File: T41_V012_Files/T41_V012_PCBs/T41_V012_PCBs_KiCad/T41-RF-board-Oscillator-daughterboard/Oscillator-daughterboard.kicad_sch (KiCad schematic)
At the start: 26 parts, among them J2 pin header, J3 pin header, J4 pin header, J5 OEBSSEN, U1 Si5351A-B-GM, U2 SY10EP51VKG, U3 SY10EP51VKG, U4 SY10EP51VKG, U5 SY10EP51VKG, U6 SY10EP51VKG, Y1 ECS-TX053-S3

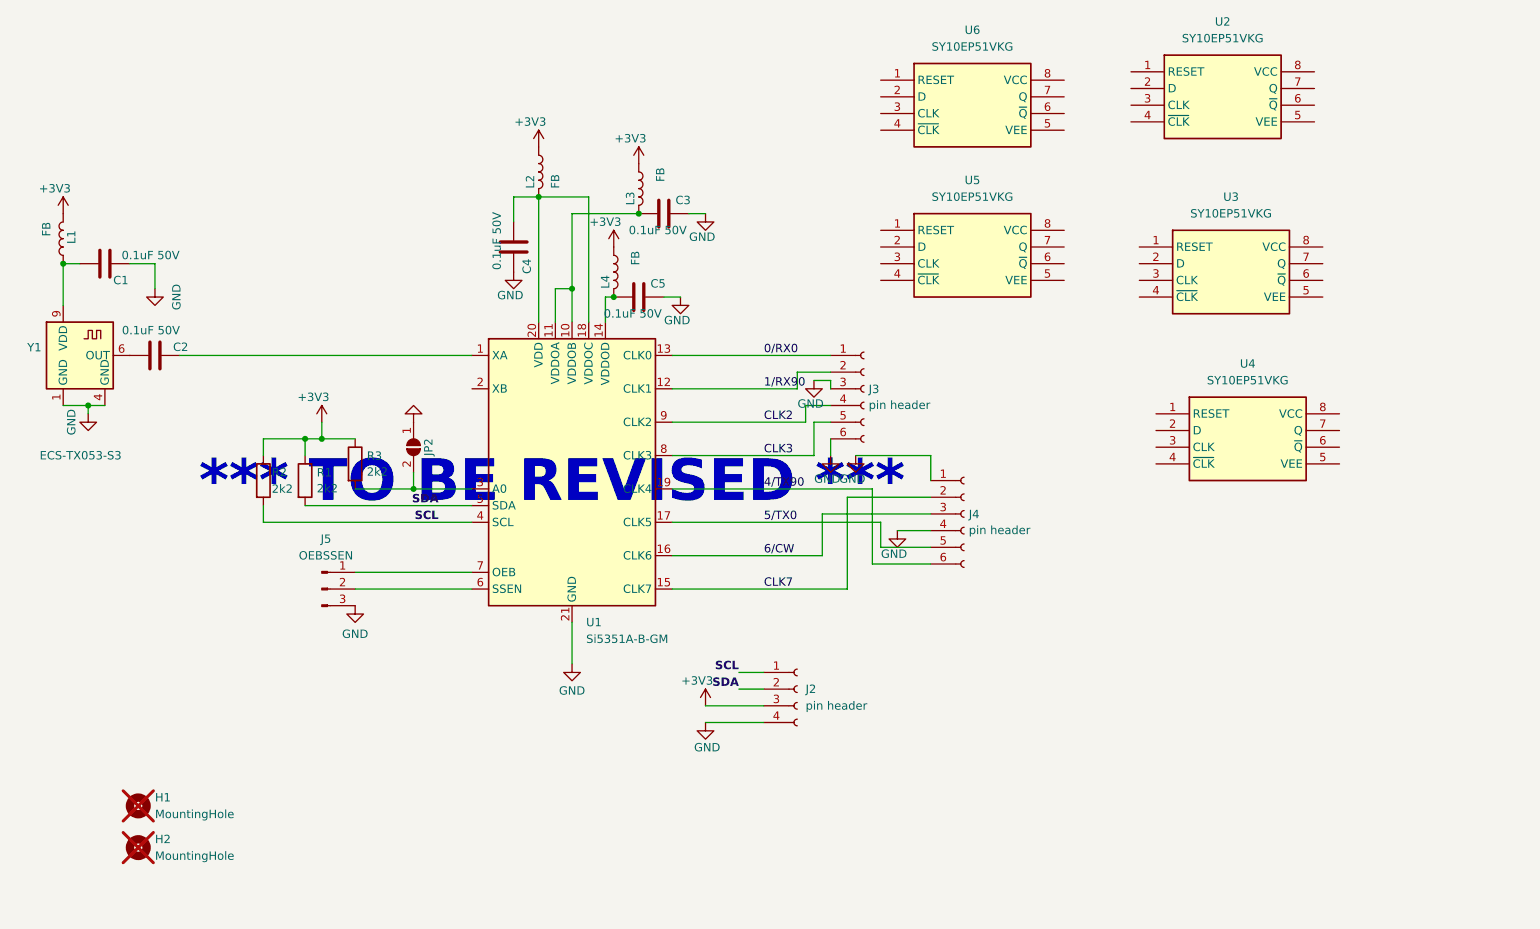
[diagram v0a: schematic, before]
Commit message: File updates
file updates
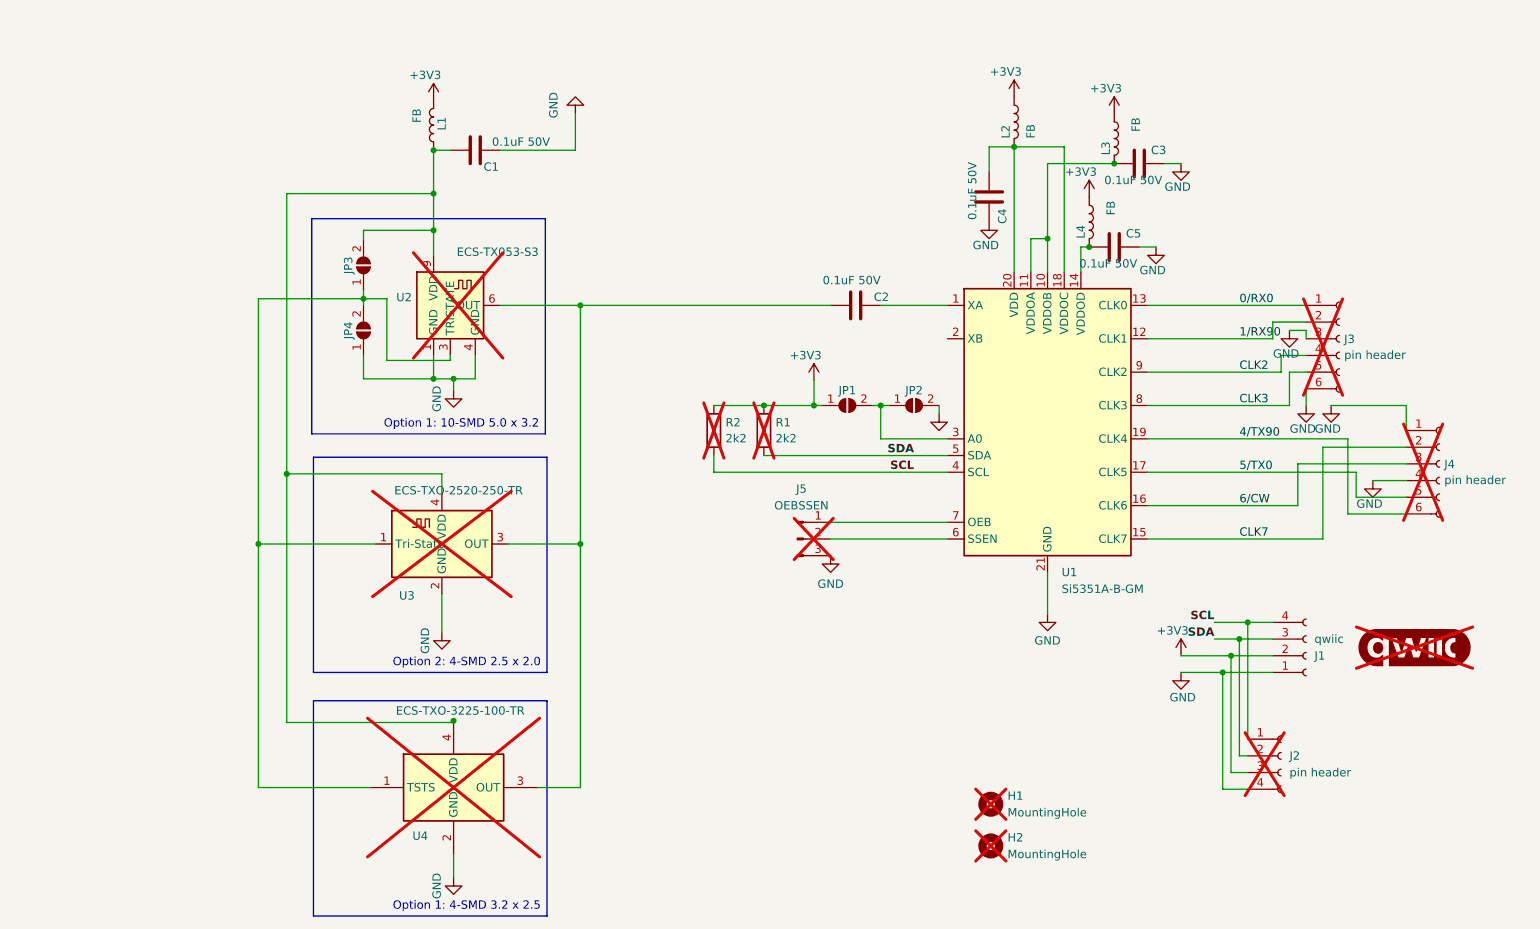
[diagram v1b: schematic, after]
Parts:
- removed R3: 2k2, Resistor_SMD:R_0603_1608Metric, symbol Device:R
- removed U2, U3, U4, U5, U6: SY10EP51VKG, T41_Library:SOP65P490X110-8N, symbol SY10EP51VKG:SY10EP51VKG
- added G1: qwiic_Logo, SparkFun-Qwiic:qwiic_4mm, symbol SparkFun-Qwiic:qwiic_Logo
- added J1: qwiic, Connector_JST:JST_SH_SM04B-SRSS-TB_1x04-1MP_P1.00mm_Horizontal, symbol Connector:Conn_01x04_Socket
- added JP1, JP3, JP4: SolderJumper_2_Open, Jumper:SolderJumper-2_P1.3mm_Open_TrianglePad1.0x1.5mm, symbol Jumper:SolderJumper_2_Open
- added U3: ECS-TXO-2520-250-TR, Oscillator:Oscillator_SMD_ECS_2520MV-xxx-xx-4Pin_2.5x2.0mm, symbol Oscillator:ECS-2520MV-xxx-xx
- added U4: ECS-TXO-3225-100-TR, ECSTXO3225120TR, symbol ECS-TXO-3225-100-TR:ECS-TXO-3225-100-TR
- J2, J5, R1, R2: now not fitted; now left out of the parts list
- J3, J4: now not fitted
- JP2: now left out of the parts list
- U2: renamed from Y1; now not fitted; now left out of the parts list
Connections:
- net +3V3: now also J1.2 (Pin_2), JP1.1 (A)
- net GND: now also JP2.2 (B), J1.1 (Pin_1), JP4.1 (A), U3.2 (GND), U4.2 (GND); no longer JP2.1 (A)
- net SCL: now also J1.4 (Pin_4)
- net SDA: now also J1.3 (Pin_3)
- net at C2.2, U2.6 (OUT): now also U3.3 (OUT), U4.3 (OUT)
- net at C1.1, L1.1, U2.9 (VDD): now also JP3.2 (B), U3.4 (VDD), U4.4 (VDD)
- net at U1.3 (A0): now also JP2.1 (A), JP1.2 (B); no longer JP2.2 (B)
- new net: JP3.1 (A), JP4.2 (B), U2.3 (TRISTATE), U3.1 (Tri-State), U4.1 (TSTS)
- no-connect marks 0 -> 1
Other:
- note removed: "*** TO BE REVISED ***"
- company: Designed by WJ Schmidt - K9HZ -> WJ Schmidt - K9HZ
- title: Si5341A-D-GM Daughter Board -> T41 V12.7 Oscillator Daughter Board
- moved on the sheet: C1, C2, C3, C4, C5, H1, H2, JP2, L1, L2, L3, L4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
